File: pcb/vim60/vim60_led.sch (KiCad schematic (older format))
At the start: 62 parts

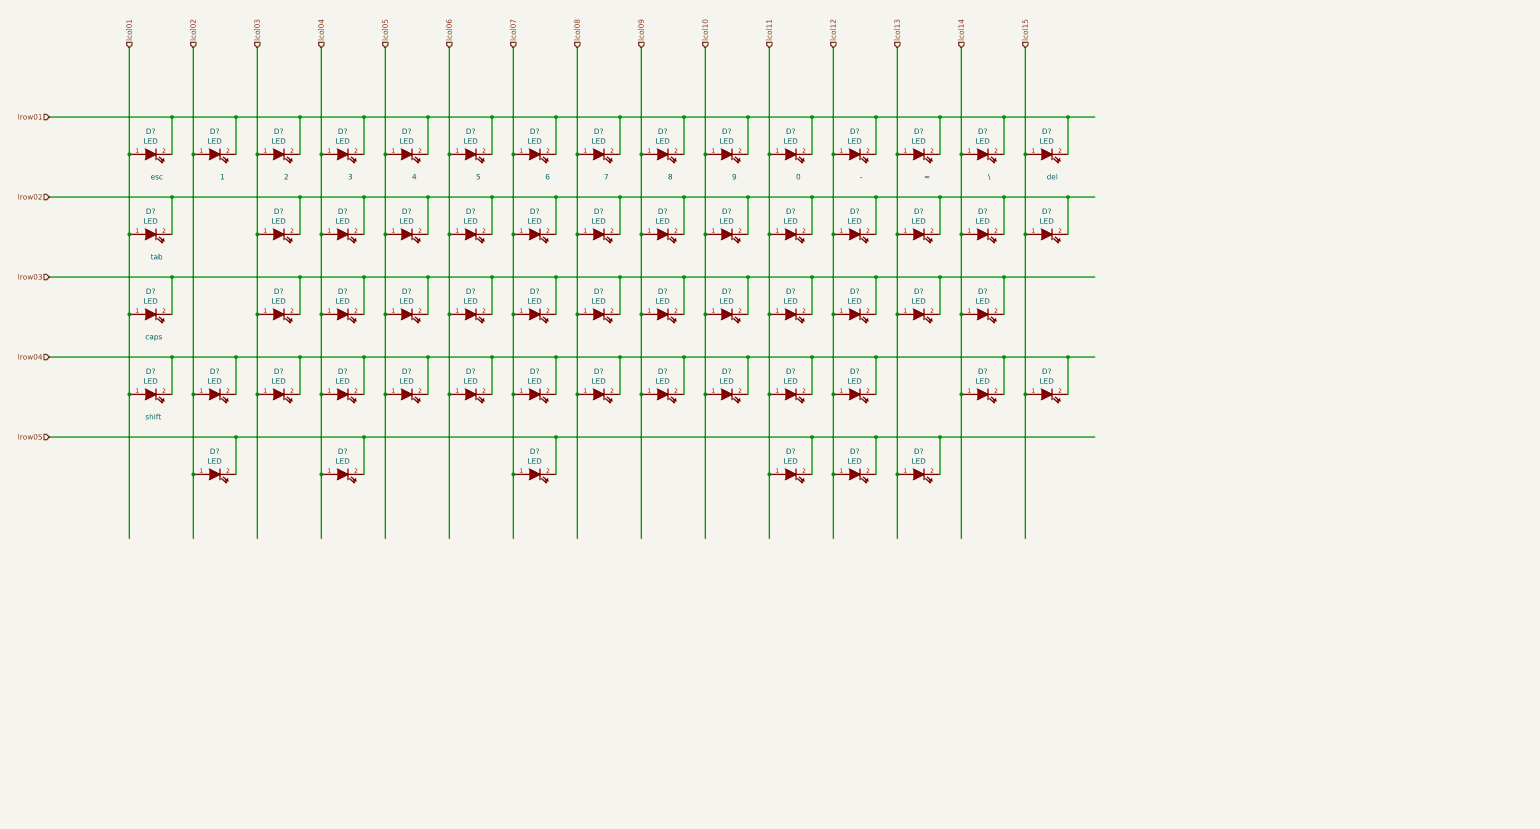
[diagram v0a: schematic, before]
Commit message: 200517
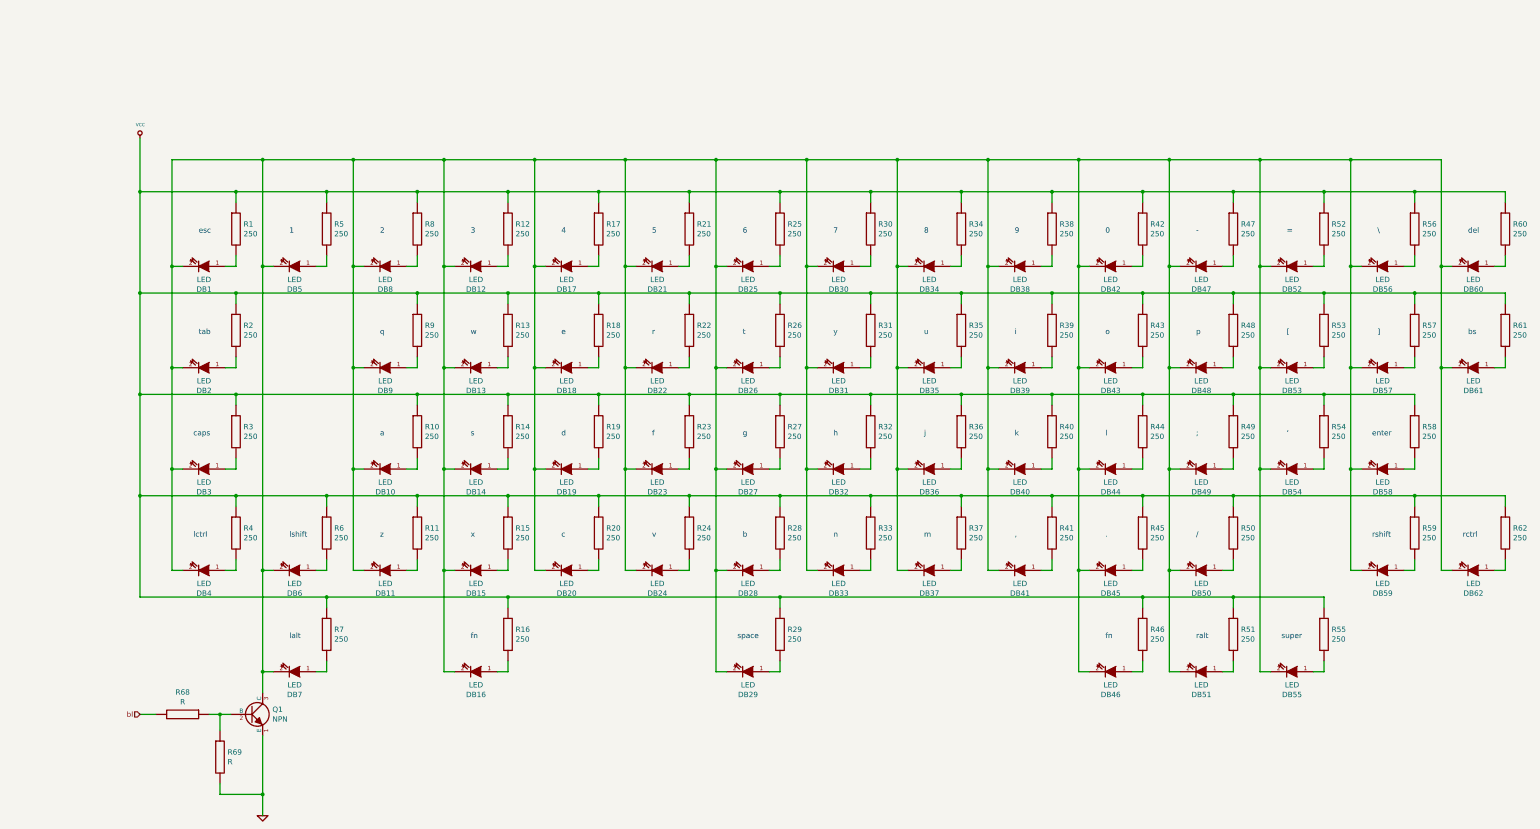
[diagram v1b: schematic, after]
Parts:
- removed D? (x61): LED, symbol device:LED
- added DB10, DB11, DB12, DB13, DB14, DB15, DB16, DB17, DB18, DB19, DB2, DB20, DB21, DB22, DB23, DB24, DB25, DB26, DB27, DB28, DB29, DB3, DB30, DB31, DB32, DB33, DB34, DB35, DB36, DB37, DB38, DB39, DB4, DB40, DB41, DB42, DB43, DB44, DB45, DB46, DB47, DB48, DB49, DB5, DB50, DB51, DB52, DB53, DB54, DB55, DB56, DB57, DB58, DB59, DB6, DB60, DB61, DB62, DB7, DB8, DB9: LED, mx1a:MX1A-led, symbol device:LED
- added Q1: NPN, device:2SC5866, symbol device:NPN
- added R1, R10, R11, R12, R13, R14, R15, R16, R17, R18, R19, R2, R20, R21, R22, R23, R24, R25, R26, R27, R28, R29, R3, R30, R31, R32, R33, R34, R35, R36, R37, R38, R39, R4, R40, R41, R42, R43, R44, R45, R46, R47, R48, R49, R5, R50, R51, R52, R53, R54, R55, R56, R57, R58, R59, R6, R60, R61, R62, R7, R8, R9: 250, 0805:0805R, symbol device:R
- added R68, R69: R, 0805:0805R, symbol device:R
- DB1: renamed from D?; footprint (none) -> mx1a:MX1A-led
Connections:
- net labels added: GND, VCC, bl
- net labels removed: lcol01, lcol02, lcol03, lcol04, lcol05, lcol06, lcol07, lcol08, lcol09, lcol10, lcol11, lcol12, lcol13, lcol14, lcol15, lrow01, lrow02, lrow03, lrow04, lrow05
- wire segments 206 -> 400
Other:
- note added: ","
- note added: "."
- note added: "/"
- note added: ";"
- note added: "["
- note added: "]"
- note added: "a"
- note added: "b"
- note added: "bs"
- note added: "c"
- note added: "d"
- note added: "e"
- note added: "enter"
- note added: "f"
- note added: "fn"
- note added: "g"
- note added: "h"
- note added: "i"
- note added: "j"
- note added: "k"
- note added: "l"
- note added: "lalt"
- note added: "lctrl"
- note added: "lshift"
- note added: "m"
- note added: "n"
- note added: "o"
- note added: "p"
- note added: "q"
- note added: "r"
- note added: "ralt"
- note added: "rctrl"
- note added: "rshift"
- note added: "s"
- note added: "space"
- note added: "super"
- note added: "t"
- note added: "u"
- note added: "v"
- note added: "w"
- note added: "x"
- note added: "y"
- note added: "z"
- note added: "‘"
- note removed: "shift"
- moved on the sheet: DB1
